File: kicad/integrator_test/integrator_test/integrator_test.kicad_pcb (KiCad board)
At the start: 2 copper layers, 52.3 x 48.3 mm, 35 parts, among them J1 Conn_01x03_Pin, J2 Conn_01x02_Pin, J3 Conn_01x04_Pin, J4 Conn_01x04_Pin, J5 Conn_01x06_Pin, SW1 SW_SPDT, U1 OPA189, U2 OPA189, U3 DG419DY-T1-E3, U4 MCP45HV51-ST, U5 DG408DQ-T1-E3

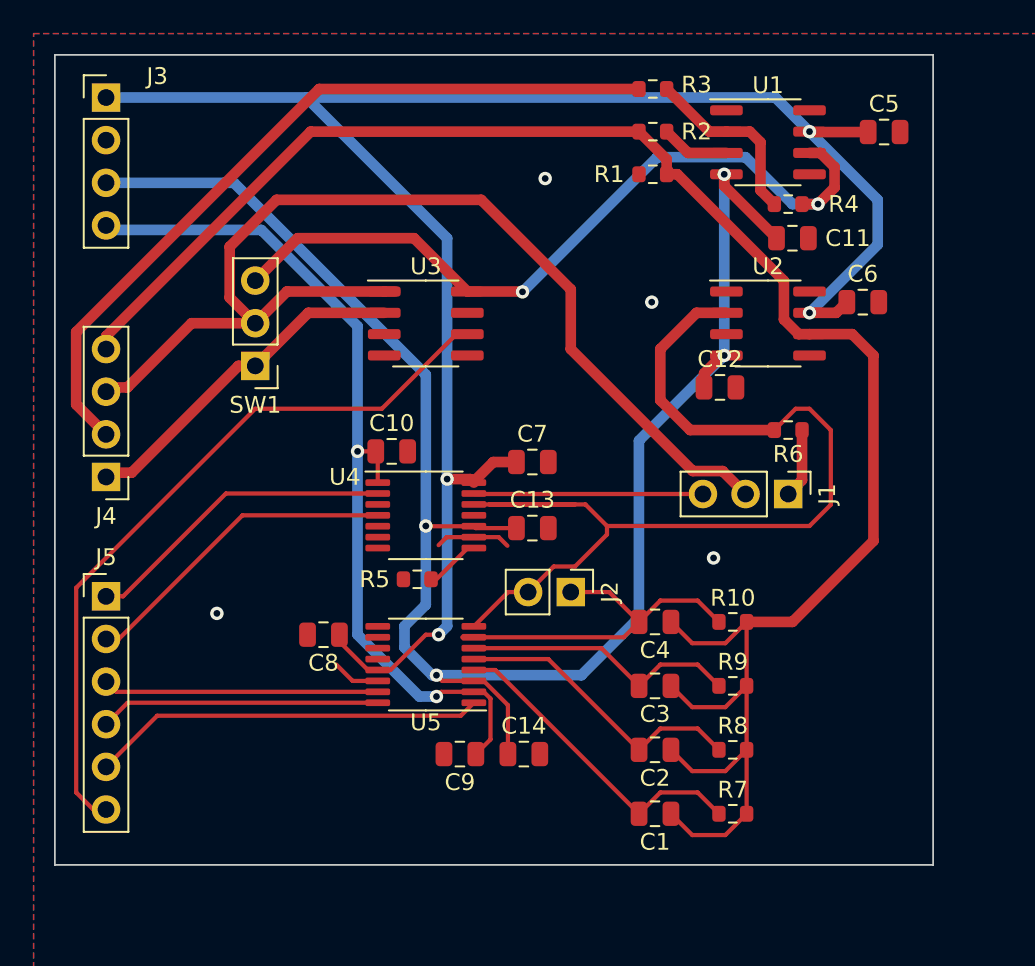
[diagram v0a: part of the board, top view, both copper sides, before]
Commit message: integrator test board v2
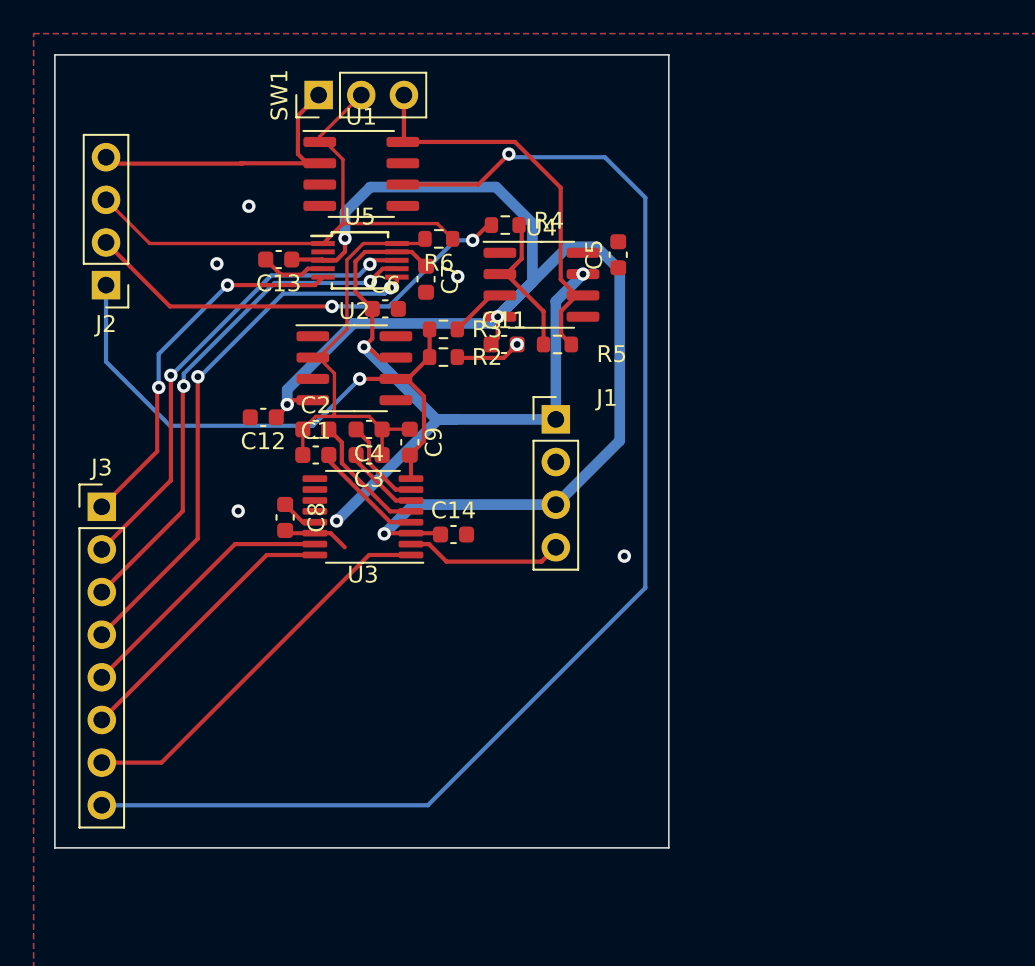
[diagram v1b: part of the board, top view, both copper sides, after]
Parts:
- removed C10: 100nF, Capacitor_SMD:C_0805_2012Metric
- removed the J1 at (61.5, 42.7)
- removed the J2 at (48.5, 48.5)
- removed J5: Conn_01x06_Pin, Connector_PinHeader_2.54mm:PinHeader_1x06_P2.54mm_Vertical
- removed R10, R7, R8, R9: 10M, Resistor_SMD:R_0603_1608Metric
- removed the R5 at (39.4, 47.8)
- removed the U4 at (39.9, 43.9)
- added J3: Conn_01x08_Pin, Connector_PinHeader_2.54mm:PinHeader_1x08_P2.54mm_Vertical, F.Cu at (20.6, 43.4)
- added U5: AD5290, Package_SO:MSOP-10_3x3mm_P0.5mm, F.Cu at (36.0, 28.7)
- C1, C11, C12, C13, C14, C2, C3, C4, C5, C6, C7, C8: footprint Capacitor_SMD:C_0805_2012Metric -> Capacitor_SMD:C_0603_1608Metric
- C9: value 100nF -> DNP; footprint Capacitor_SMD:C_0805_2012Metric -> Capacitor_SMD:C_0603_1608Metric
- moved J1 33.0 mm to (47.6, 38.2)
- moved C1 29.4 mm to (33.3, 40.3), turned to 0 degrees
- moved C6 28.5 mm to (37.5, 31.6)
- moved C2 27.8 mm to (33.3, 38.8), turned to 0 degrees
- moved C12 27.3 mm to (30.2, 38.1), turned to 180 degrees
- moved U2 24.8 mm to (35.6, 35.2)
- moved R6 23.7 mm to (40.7, 27.5)
- moved C13 22.0 mm to (31.1, 28.7), turned to 180 degrees
- moved C3 21.9 mm to (36.5, 40.3)
- moved C4 20.5 mm to (36.5, 38.8)
- moved C9 18.8 mm to (38.9, 39.6), turned to -90 degrees
- moved C11 18.3 mm to (44.5, 33.8)
- moved C5 17.4 mm to (51.3, 28.4), turned to 90 degrees
- moved R3 17.2 mm to (40.9, 32.9)
- moved SW1 16.6 mm to (33.5, 18.9), turned to 90 degrees
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- renumbered J3 to J1, J4 to J2, R1 to R2, R2 to R3, R3 to R4, R4 to R5, U3 to U1, U5 to U3, U1 to U4
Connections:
- C1 pad 1: I_OUT -> INT_R-
- C2 pad 1: I_OUT -> INT_R-
- C3 pad 1: I_OUT -> INT_R-
- C4 pad 1: I_OUT -> INT_R-
- C9 pad 1: +3V3 -> INT_R-
- C9 pad 2: GND -> I_OUT
- J2 pad 1: I_IN -> I_OUT
- J2 pad 4: I_OUT -> I_IN
- R6 pad 1: Net-(J1-Pin_1) -> INT_R+
- U3 pad 8: INT_R- -> I_OUT
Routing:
- net I_OUT: track 113.2 -> 36.2 mm, vias 0 -> 1
- net +12V: track 111.3 -> 47.0 mm, vias 4 -> 3
- net +3V3: track 52.2 -> 9.41 mm, vias 2 -> 0
- net INT_R-: track 62.4 -> 26.1 mm
- net I_OVERRIDE_EN: track 44.0 -> 77.3 mm, vias 0 -> 1
- net INT_R+: track 66.6 -> 33.4 mm
- net R_CLK: track 0.00 -> 32.4 mm, vias 0 -> 2
- net R_SDI: track 0.00 -> 30.7 mm, vias 0 -> 2
- net R_SDO: track 0.00 -> 28.8 mm, vias 0 -> 2
- net R_CS: track 0.00 -> 22.2 mm, vias 0 -> 2
- net Net-(SW1-C): track 45.7 -> 24.1 mm, vias 2 -> 0
- net -12V: track 106.1 -> 84.8 mm
- net I_OVERRIDE: track 46.4 -> 26.7 mm, vias 0 -> 2
- net R_SDA: track 19.2 -> 0.00 mm
- net R_SCL: track 18.7 -> 0.00 mm
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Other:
- board size 52.3 x 48.3 mm -> 36.6 x 47.2 mm
